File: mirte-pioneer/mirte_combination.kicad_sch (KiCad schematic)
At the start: 50 parts, among them J1 Servo3, J10 IR1, J11 Conn_01x13_Female, J12 IR Object Detector 1, J14 IR2, J17 MC1, J18 MC2, J19 Servo1, J2 Conn_01x20_Female, J20 SRF1, J21 ENC2, J23 MC1-A, J24 MC1-B, J25 SRF2, J26 ENC1, J27 Servo2, J28 I2C2, J3 Servo4, J30 I2C1, J33 line out left, J34 Power in, J35 Power out, J37 on/off, J4 Conn_01x20_Female, J5 Conn_01x06_Pin, J7 Keypad, J8 Conn_01x06_Female, J9 IR Object Detector 2, Q1 DMG2305UX, Q2 DMN2050L, SW1 on/off, U1 CH340C, U2 CH340E

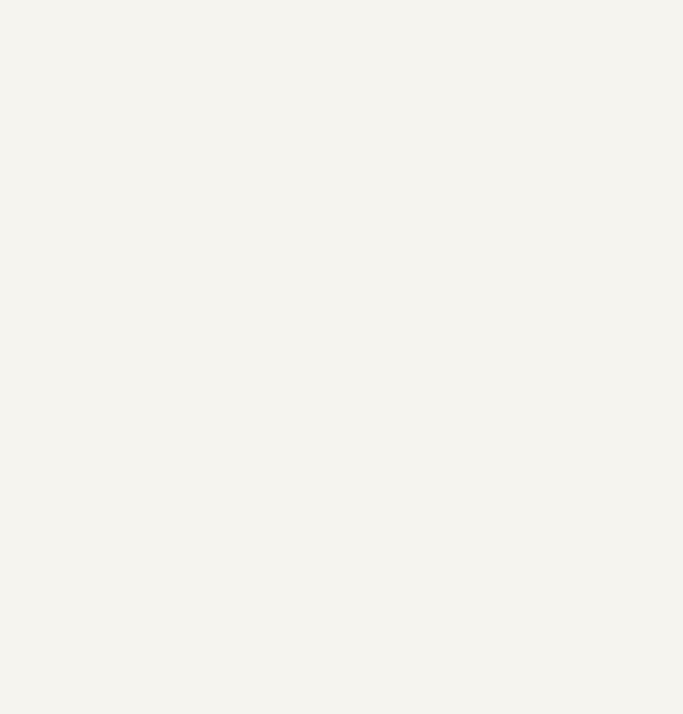
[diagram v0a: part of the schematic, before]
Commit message: test usb c pioneer pcb
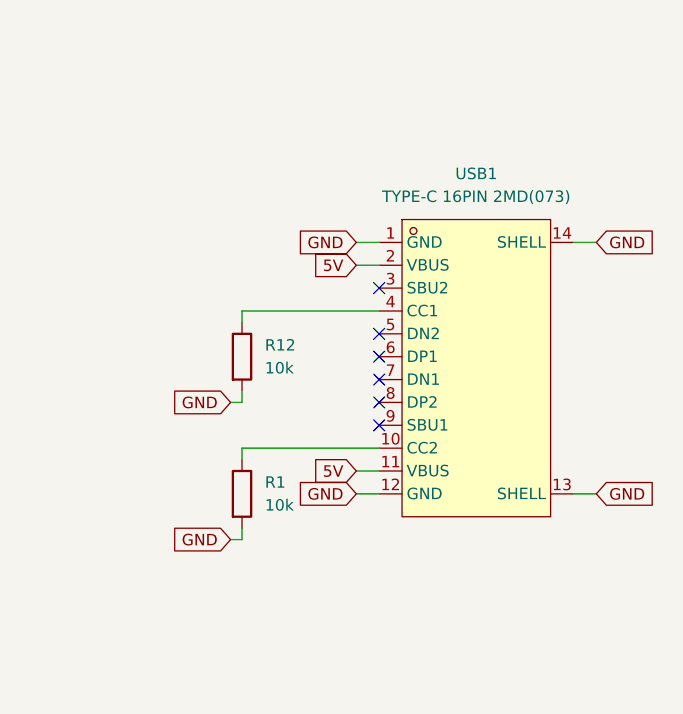
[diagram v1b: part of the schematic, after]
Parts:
- added R1, R12: 10k, Resistor_SMD:R_1206_3216Metric, symbol Device:R
- added USB1: TYPE-C 16PIN 2MD(073), lcsc:USB-C-SMD_TYPE-C-6PIN-2MD-073, symbol lcsc:TYPE-C16PIN2MD(073)
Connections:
- net 5V: now also USB1.11 (VBUS), USB1.2 (VBUS)
- net GND: now also R1.2, R12.2, USB1.1 (GND), USB1.12 (GND), USB1.13 (SHELL), USB1.14 (SHELL)
- new net: R1.1, USB1.10 (CC2)
- new net: R12.1, USB1.4 (CC1)
- no-connect marks 21 -> 27
